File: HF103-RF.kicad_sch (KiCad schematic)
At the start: 28 parts, among them T2 ETC1-1T-2TR, U2 74CBTLV3253, U5 LTC6400CUD-20-PBF

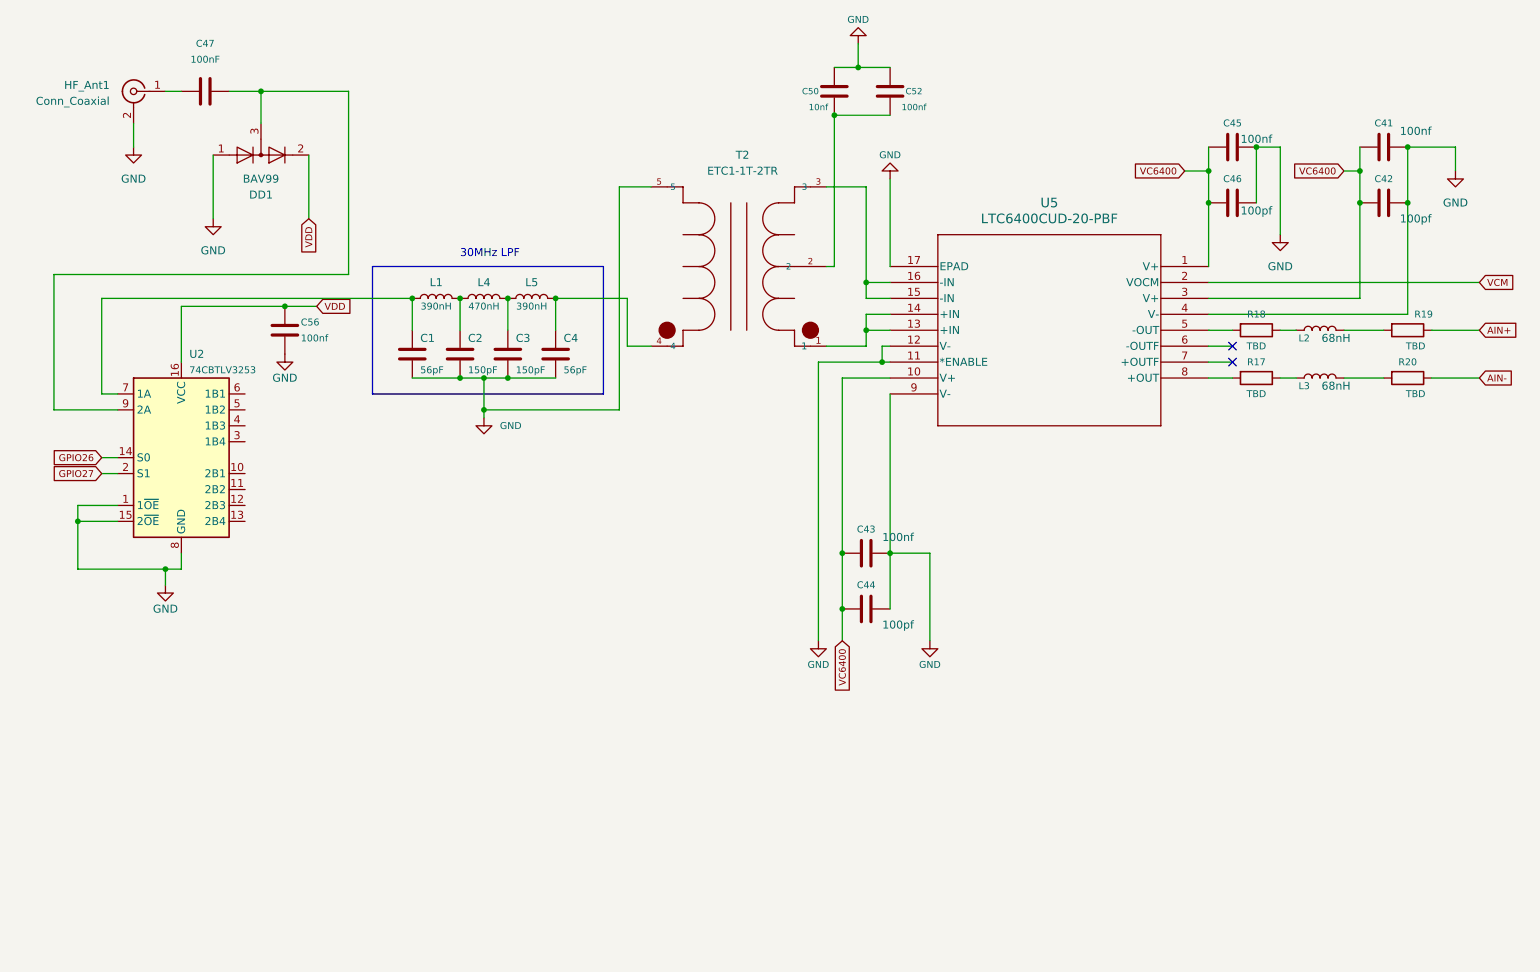
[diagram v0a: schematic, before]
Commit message: Commit latest schematic changes
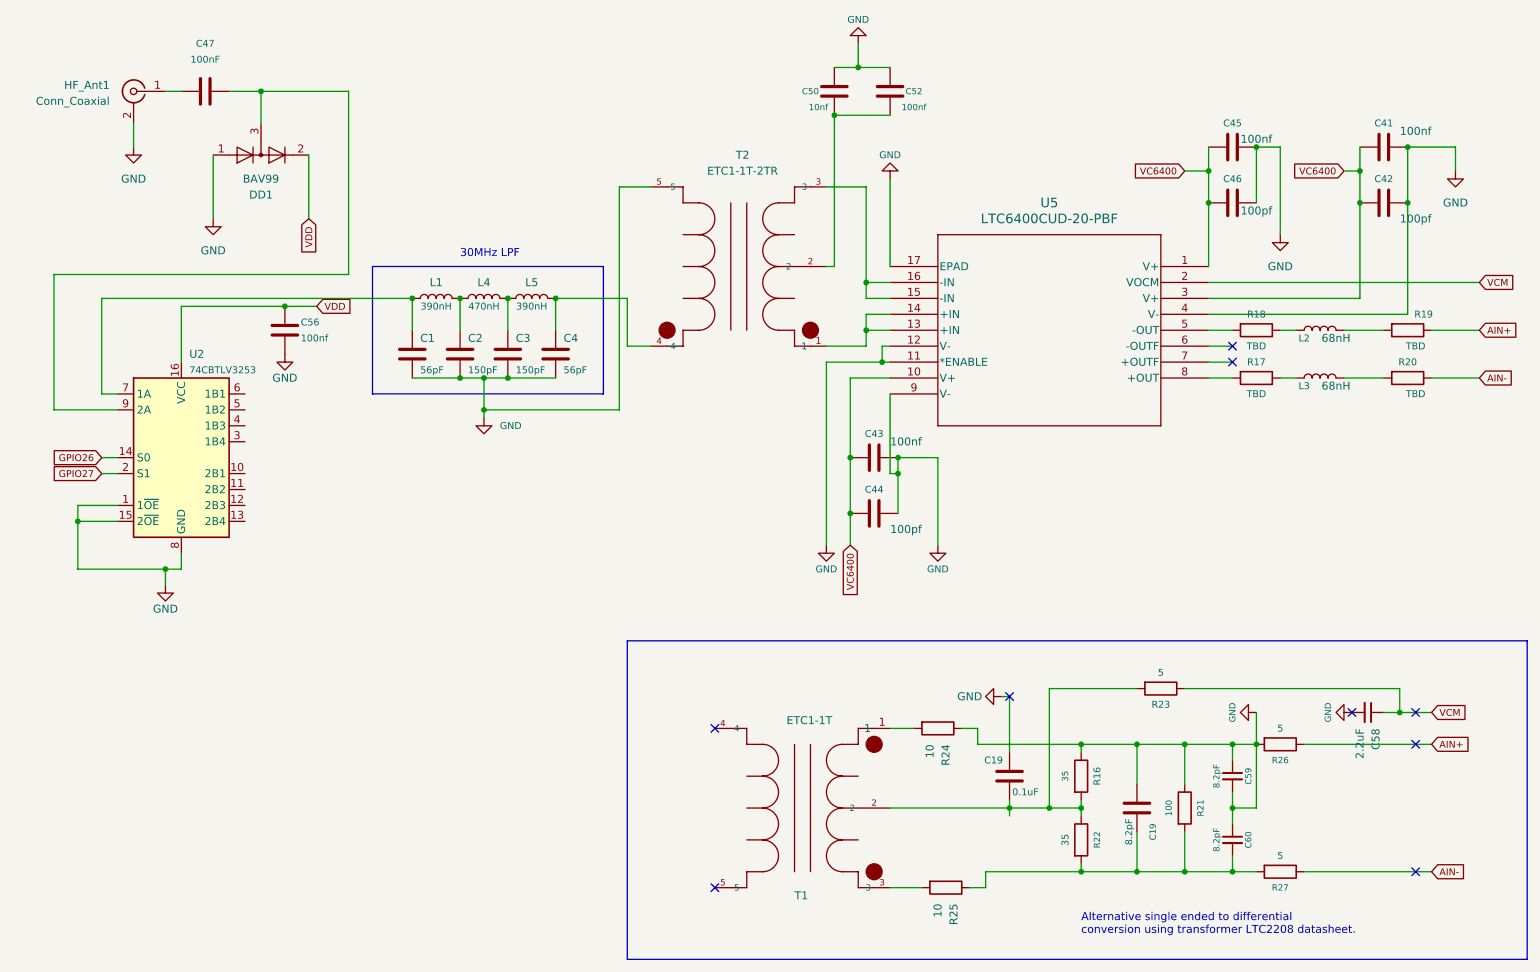
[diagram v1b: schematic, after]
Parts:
- added C19: 8.2pF, Capacitor_SMD:C_0805_2012Metric_Pad1.18x1.45mm_HandSolder, symbol Device:C
- added C19: 0.1uF, Capacitor_SMD:C_0805_2012Metric_Pad1.18x1.45mm_HandSolder, symbol Device:C
- added C58: 2.2uF, symbol Device:C_Small
- added C59, C60: 8.2pF, symbol Device:C_Small
- added R16, R22: 35, Resistor_SMD:R_0612_1632Metric, symbol Device:R
- added R21: 100, Resistor_SMD:R_0612_1632Metric, symbol Device:R
- added R23, R26, R27: 5, Resistor_SMD:R_0612_1632Metric, symbol Device:R
- added R24, R25: 10, Resistor_SMD:R_0805_2012Metric_Pad1.20x1.40mm_HandSolder, symbol Device:R
- added T1: ETC1-1T, E_SERIES_1, symbol HF103-redux:ETC1-1T-2TR
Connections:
- net AIN+: now also R26.1
- net AIN-: now also R27.1
- net GND: now also C19.1, C19.1, C58.2, C59.1, C59.2, C60.1, R16.1, R21.1, R24.1, R26.2
- net VCM: now also C58.1, R23.1
- new net: C19.2, C60.2, R21.2, R22.2, R25.1, R27.2
- new net: C19.2, R16.2, R22.1, R23.2, T1.2
- new net: R24.2, T1.1
- new net: R25.2, T1.3
- no-connect marks 2 -> 9
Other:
- note added: "Alternative single ended to differential conversion using transformer LTC2208 datasheet."
- moved on the sheet: C43, C44
